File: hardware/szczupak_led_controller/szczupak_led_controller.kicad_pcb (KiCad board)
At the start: 4 copper layers, 126 parts, among them IC1 STM32G0B1CBT6, IC2 SN65HVD230DR, IC3 TLV75533PDBVR, J1 Conn_01x05, J10 XT60PW-M, J2 USB4110-GF-A, J3 CAN_CONN, J4 43650-0200, J5 43650-0300, J6 CAN_CONN, J7 Conn_EXT, J8 XT60PW-M, J9 XT60PW-M, Q1 AO4407A, Q2 AO3401A, Q3 2N7002, Q4 2N7002, Q5 2N7002, U1 USBLC6-2SC6, U3 3568

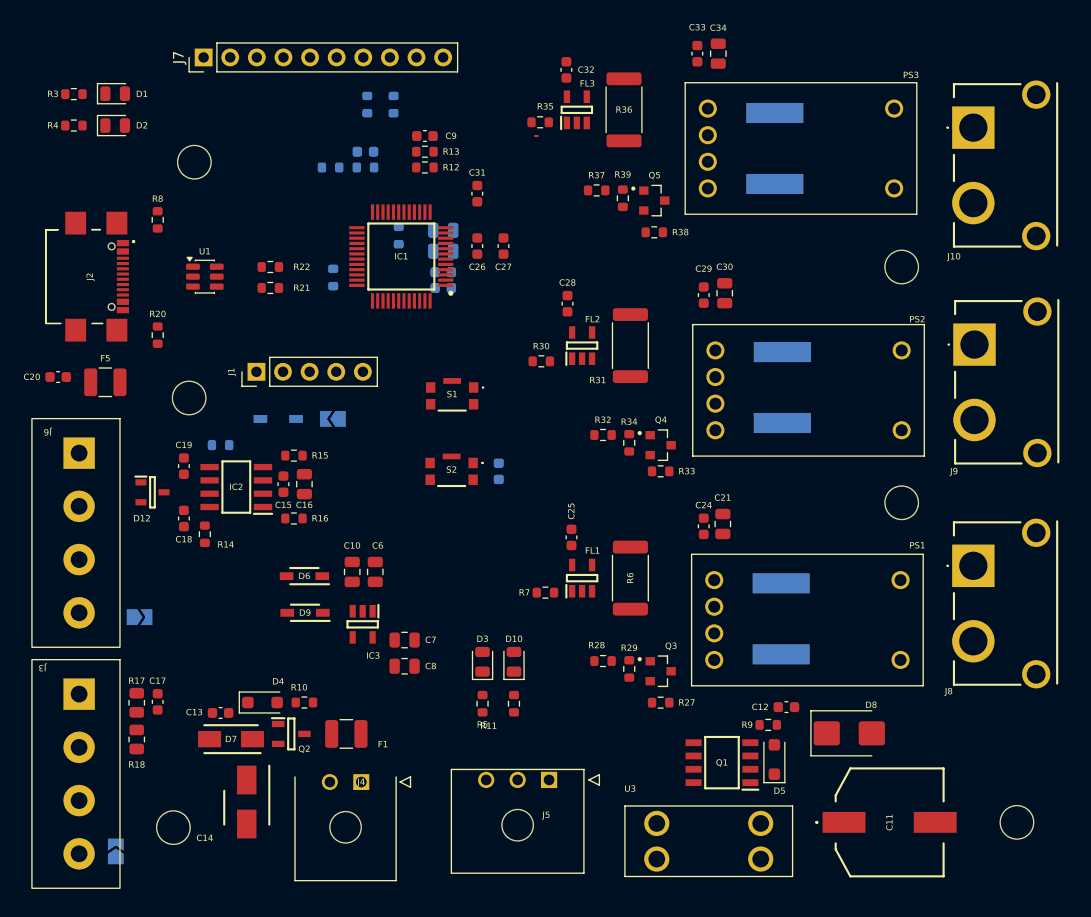
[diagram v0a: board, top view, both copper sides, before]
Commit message: #8 Added routing for usb and mcu. Started pouring of power elements
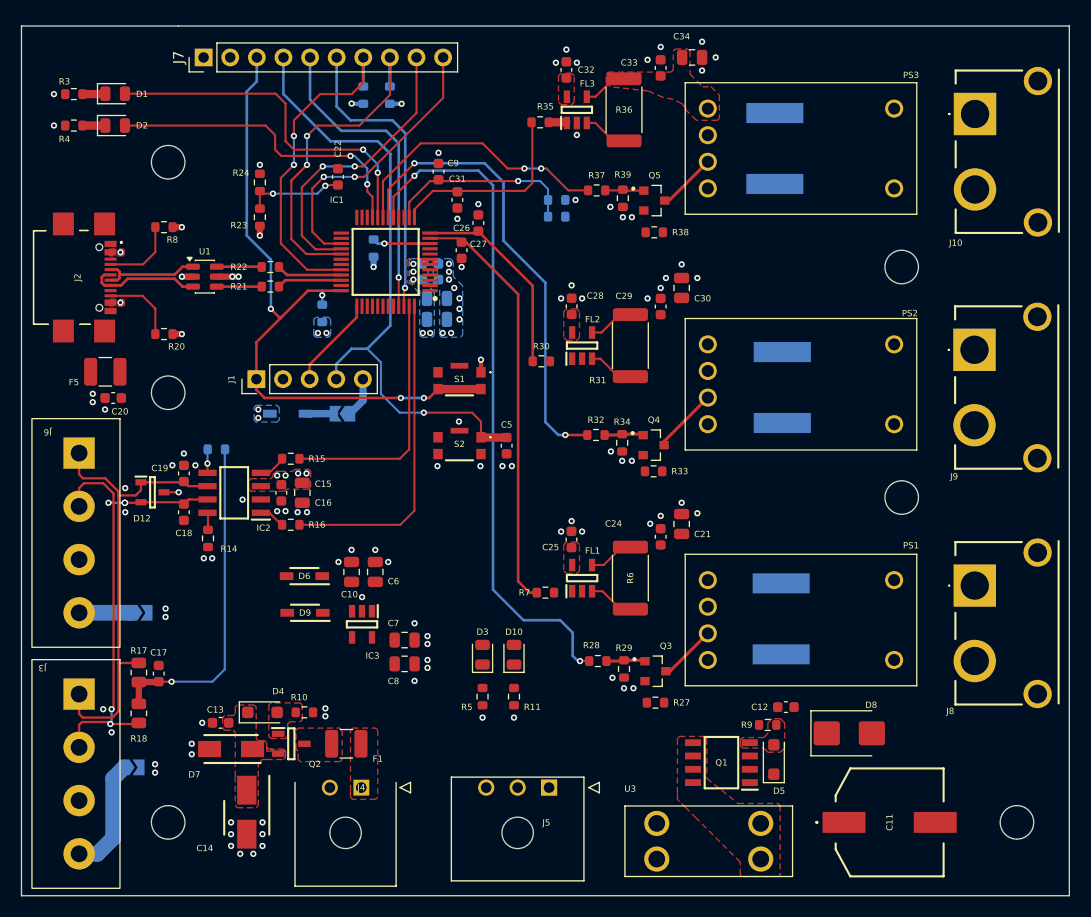
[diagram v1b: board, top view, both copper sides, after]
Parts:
- C22, C5, R23, R24: moved to F.Cu
- R12, R13: moved to B.Cu
- moved R12 13.4 mm to (120.1, 68.2)
- moved R13 13.4 mm to (120.1, 66.6)
- moved R24 10.2 mm to (91.8, 64.9), turned to -90 degrees
- moved R23 8.25 mm to (91.8, 68.2), turned to -90 degrees
- moved JP3 8.17 mm to (79.5, 120.8), turned to 0 degrees
- moved C3 6.53 mm to (108.7, 76.0)
- moved C4 6.53 mm to (108.7, 78.0)
- moved C20 5.62 mm to (77.8, 85.5)
- moved C29 4.25 mm to (130.0, 76.8)
- moved C24 4.23 mm to (130.0, 98.8)
- moved C30 4.14 mm to (132.0, 75.0)
- moved C21 3.93 mm to (132.0, 97.5)
- moved C33 3.75 mm to (130.0, 54.0)
- moved C9 3.64 mm to (108.8, 63.9), turned to 90 degrees
- moved R2 3.58 mm to (97.7, 77.4), turned to -90 degrees
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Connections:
- net Net-(D1-K) renamed /02_mcu/LED_STATUS_R
- net Net-(D2-K) renamed /02_mcu/LED_FAULT_R
- net Net-(FL1-OUT) renamed /04_power_output/ADC_R1
- net Net-(FL2-OUT) renamed /04_power_output/ADC_R2
- net Net-(FL3-OUT) renamed /04_power_output/ADC_R3
- net Net-(JP2-A) renamed /03_interfaces/CAN_SHIELD_1
- net Net-(JP3-A) renamed /03_interfaces/CAN_SHIELD_2
- net Net-(Q3-Pad1) renamed /04_power_output/PWM_LED1_GATE
- net Net-(Q4-Pad1) renamed /04_power_output/PWM_LED2_GATE
- net Net-(Q5-Pad1) renamed /04_power_output/PWM_LED3_GATE
- C15 pad 1: unconnected-(C15-Pad1) -> +3.3V
- C15 pad 2: unconnected-(C15-Pad2) -> GND
- C16 pad 1: unconnected-(C16-Pad1) -> +3.3V
- C16 pad 2: unconnected-(C16-Pad2) -> GND
- J7 pad 10: /PWM_EXT -> /GPIO_EXT
- J7 pad 9: /GPIO_EXT -> /PWM_EXT
- S1 pad 5: GND -> unconnected-(S1-GROUND-Pad5)
- S2 pad 5: GND -> unconnected-(S2-GROUND-Pad5)
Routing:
- net /NRST: track 0.00 -> 65.9 mm, vias 0 -> 2
- net /PWM_LED1: track 0.00 -> 65.1 mm, vias 0 -> 2
- net /SWCLK_BOOT0: track 0.00 -> 64.8 mm, vias 0 -> 4
- net /03_interfaces/CAN_P: track 0.00 -> 46.8 mm, vias 0 -> 5
- net /03_interfaces/CAN_N: track 0.00 -> 45.1 mm
- net /PWM_LED2: track 0.00 -> 44.5 mm, vias 0 -> 2
- net /ADC_LED1: track 0.17 -> 40.2 mm
- net /02_mcu/LED_STATUS: track 0.24 -> 34.3 mm, vias 0 -> 2
- net /I2C1_SDA: track 0.00 -> 32.3 mm, vias 0 -> 2
- net /I2C1_SCL: track 0.00 -> 31.8 mm, vias 0 -> 2
- net /03_interfaces/CAN_SPLIT: track 0.00 -> 31.3 mm, vias 0 -> 1
- net /02_mcu/LED_FAULT: track 0.00 -> 31.2 mm, vias 0 -> 2
- net /CAN_TX: track 0.00 -> 31.1 mm
- net /USART1_TX: track 0.00 -> 29.8 mm, vias 0 -> 1
- net /USART1_RX: track 0.00 -> 28.9 mm, vias 0 -> 1
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- added copper zone on B.Cu, net +3.3V
- added copper zone on F.Cu, net +3.3V
- added copper zone on F.Cu, net /01_power_input/12V_FUSE
- added copper zone on F.Cu, net /01_power_input/5V_FUSE
- added copper zone on F.Cu, net /01_power_input/5V_IN
- added copper zone on F.Cu, net /01_power_input/5V_PROT
- added copper zone on F.Cu, net /01_power_input/Q1_GATE
- added copper zone on F.Cu, net /01_power_input/Q2_GATE
- added copper zone on F.Cu, net /04_power_output/12V_CH3
- added copper zone on F.Cu, net /USB_5V
- added copper zone on B.Cu, net GND
- added copper zone on In1.Cu, net GND
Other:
- board outline added: 100 x 83 mm
